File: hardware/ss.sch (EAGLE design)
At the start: 84 parts, among them IC1 DS3231, Q1 BSS138, Q2 si2305cd, Q4 si2305cd, Q5 8MHz, Q6 si2305cd, T1 BC846, U1 SPX5205 3v3, U17 AVR_SPI_PRG_6PTH, U2 CN3083, U3 SPX5205 3v3, U5 ATMEGA328, U6 microSD Socket

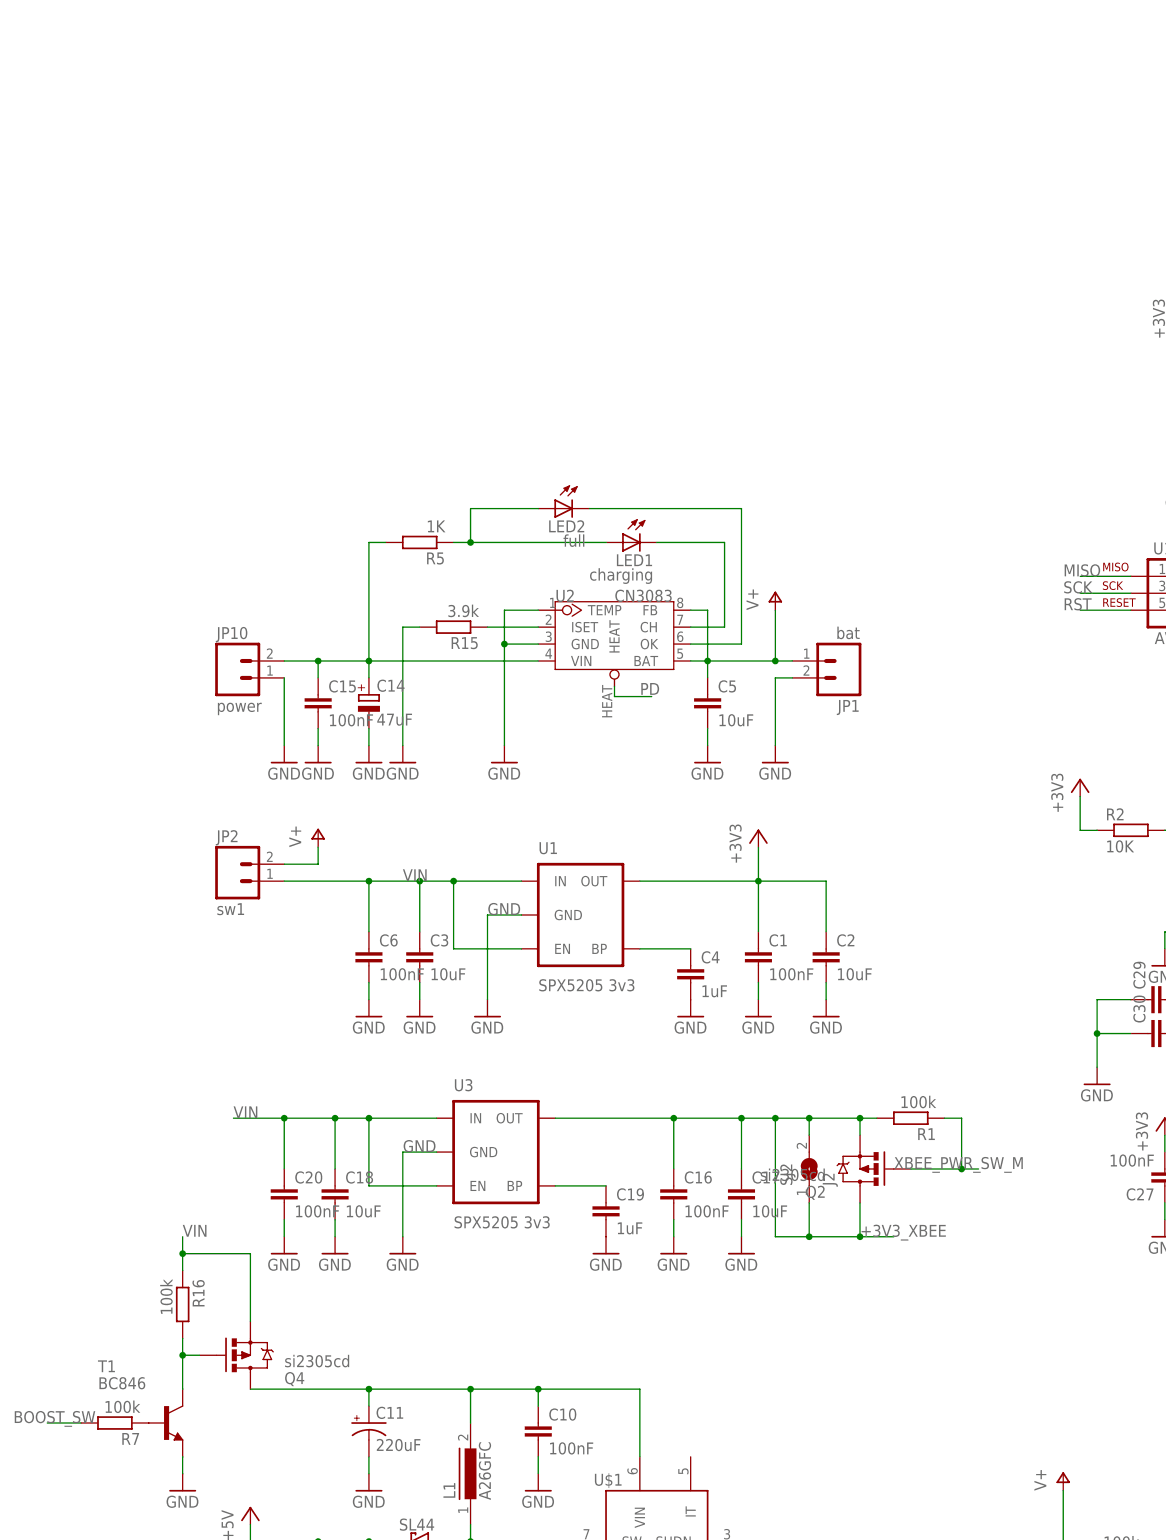
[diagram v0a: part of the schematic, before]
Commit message: hopefully flawless
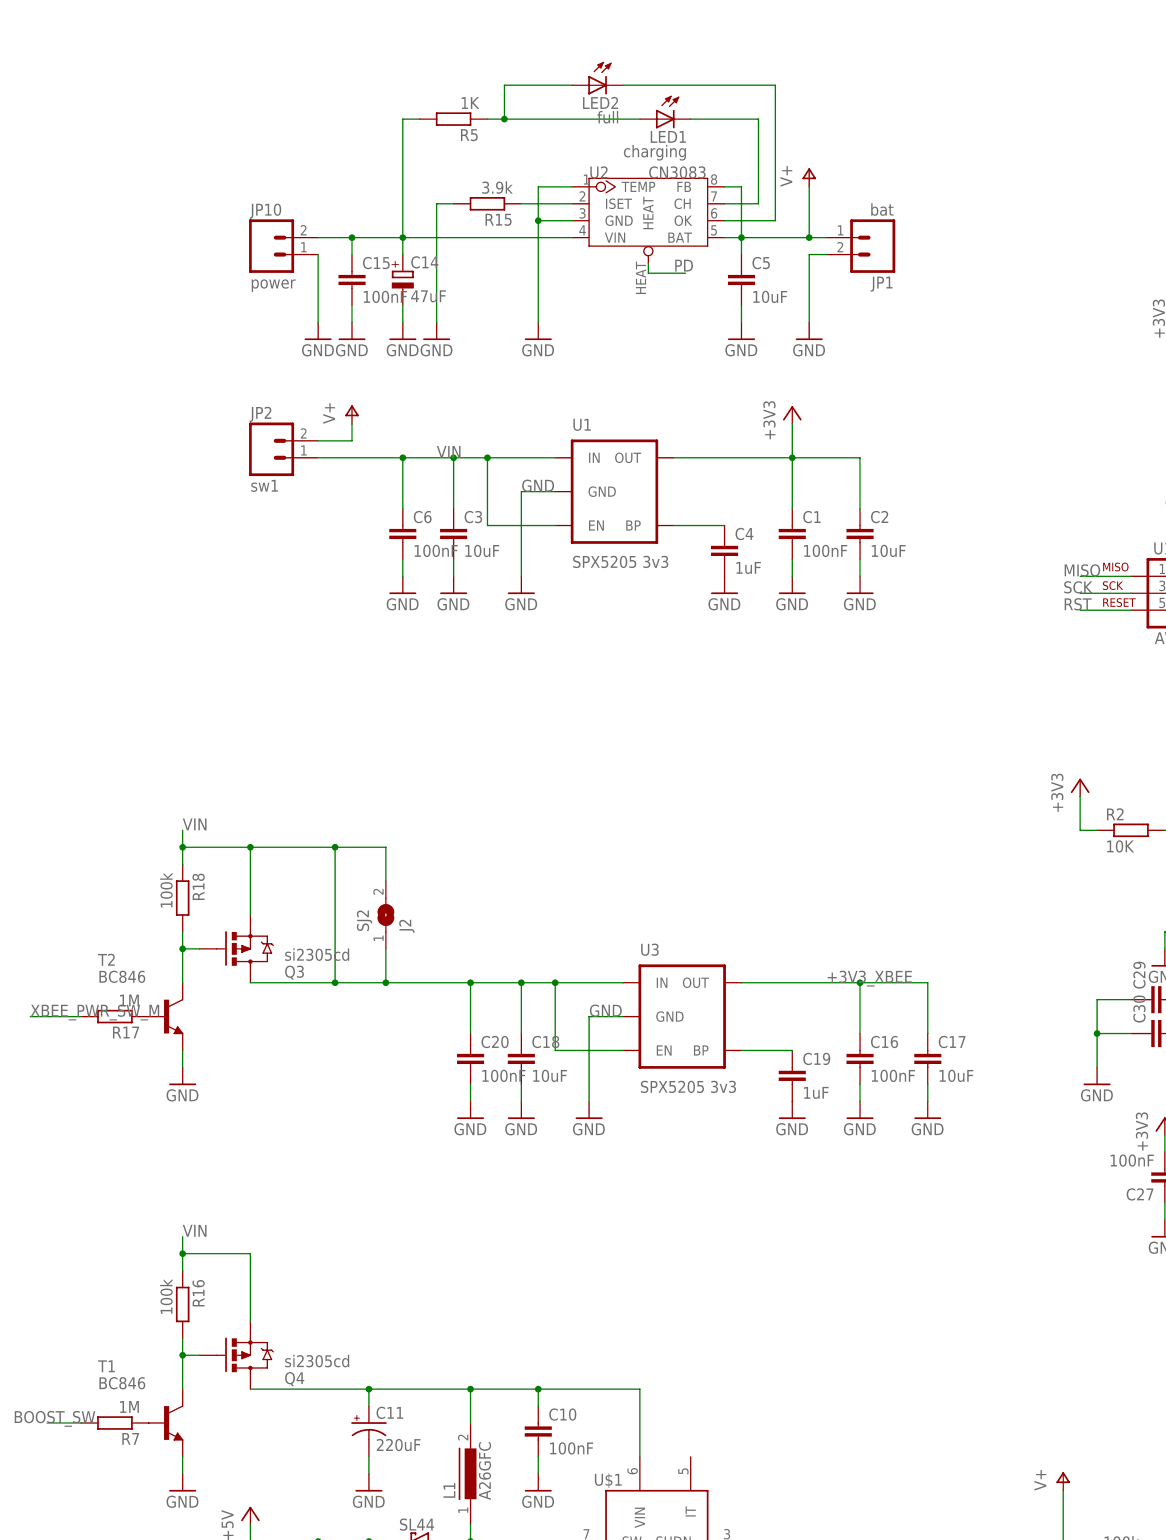
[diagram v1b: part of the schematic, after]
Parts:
- removed Q2: si2305cd, Simplex-DiscreteSemi:MOSFET-PCHANNELSMD_POWER
- removed R1: 100k, rcl:R-EU_R0805W
- added Q3: si2305cd, Simplex-DiscreteSemi:MOSFET-PCHANNELSMD_POWER
- added R17: 1M, rcl:R-EU_R0805W
- added R18: 100k, rcl:R-EU_R0805W
- added T2: BC846, transistor:BC846
- R7: value 100k -> 1M
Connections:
- new net N$18: R17.1, T2.B
- new net N$20: Q3.G, R18.2, T2.C
- net +3V3_XBEE: no longer Q2.D, Q2.S, R1.2, SJ2.1, SJ2.2
- net GND: now also T2.E
- net VIN: now also Q3.D, Q3.S, R18.1, SJ2.1, SJ2.2
- net XBEE_PWR_SW_M: now also R17.2; no longer Q2.G, R1.1
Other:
- moved on the sheet: C1, C14, C15, C16, C17, C18, C19, C2, C20, C3, C4, C5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
